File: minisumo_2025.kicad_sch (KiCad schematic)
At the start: 125 parts, among them J1 USB_C Connector, J10 DISTANCE_R90, J11 DISTANCE_R, J12 DISTANCE_RF, J13 DISTANCE_L90, J14 DISTANCE_L, J15 LINE_LEFT, J16 DISTANCE_LF, J3 START_MODULE, J4 MOTOR1, J5 MOTOR2, J6 BATT_IN, J8 DISTANCE_CENTER, J9 LINE_RIGHT, SW1 RESET, SW2 CASE, SW5 BOOT, U1 LMR33630ADDAR, U2 USBLC6-2P6, U3 ESP32-S3-WROOM-1, U4 TLV75733PDBVR, U5 TXS0108EPWR, U6 MC33926PNB, U7 MC33926PNB

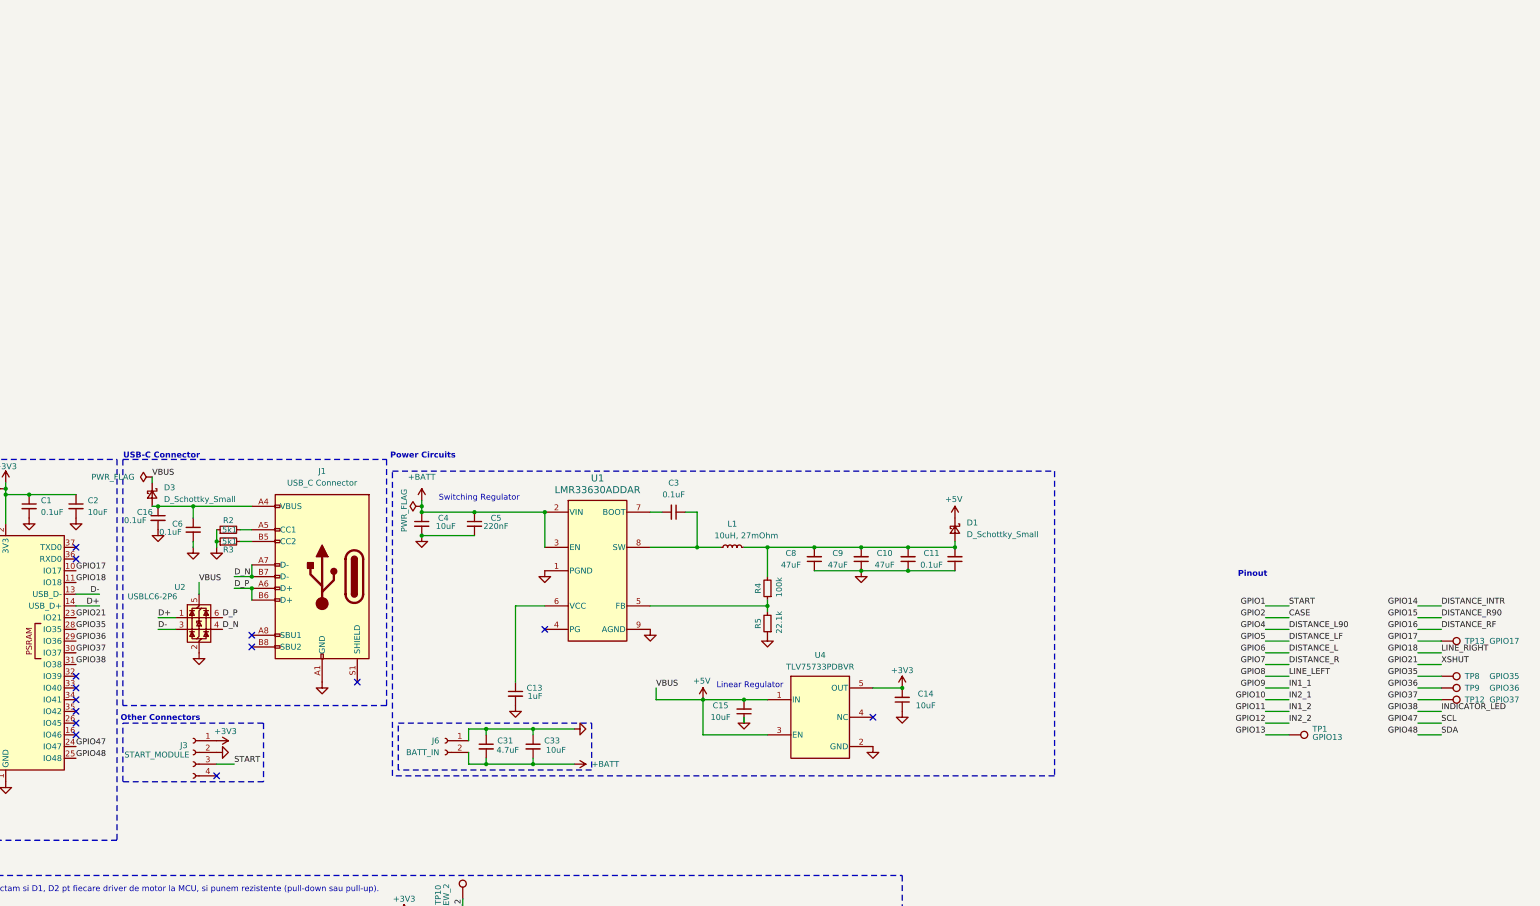
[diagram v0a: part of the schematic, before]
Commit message: final layout
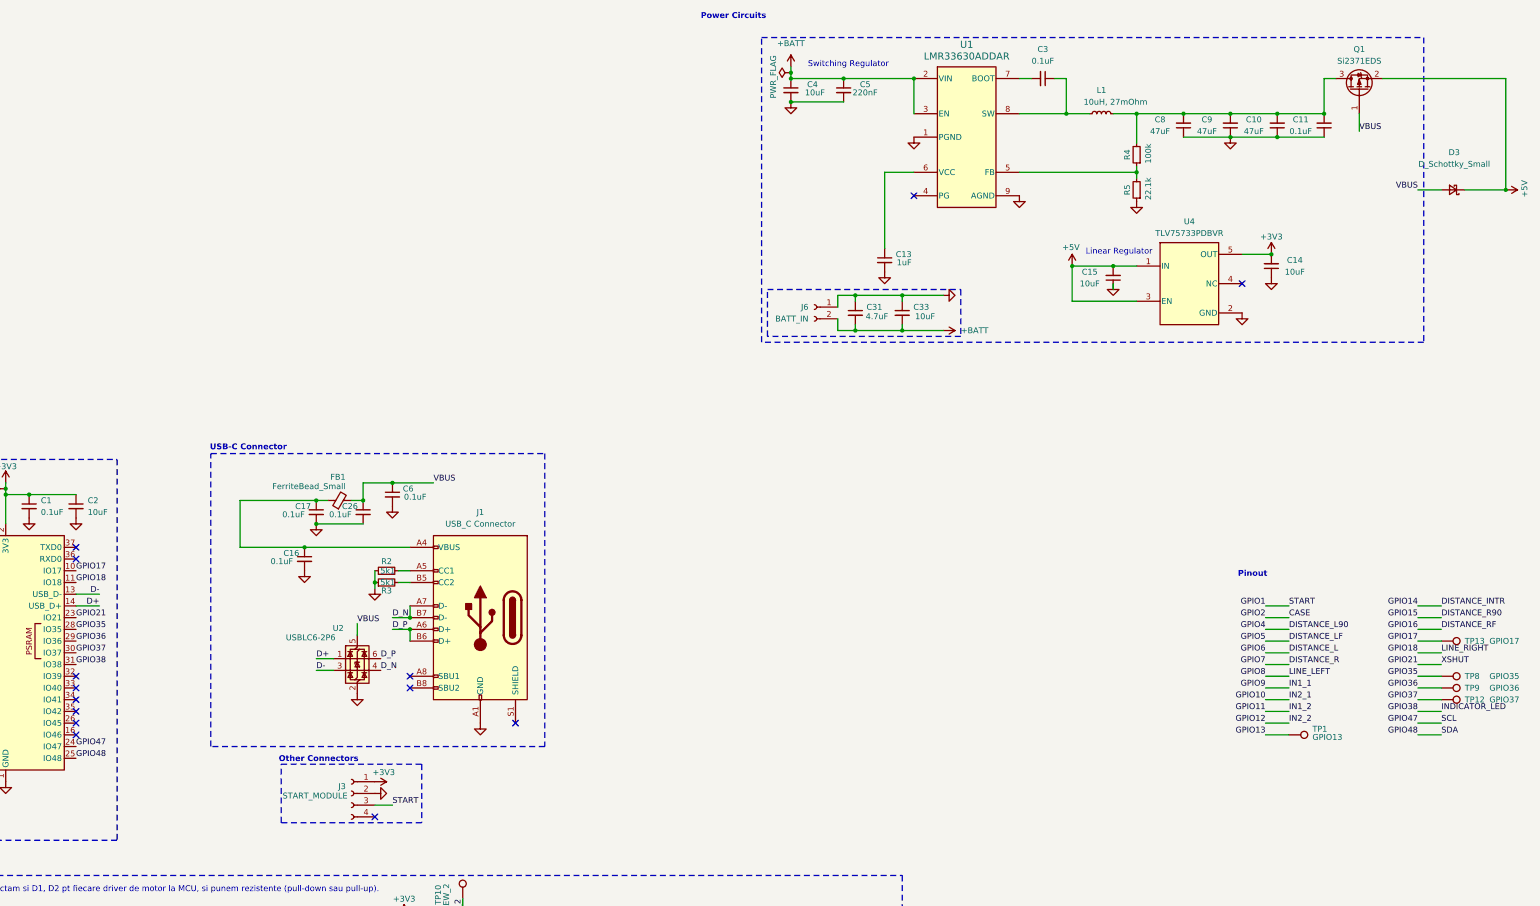
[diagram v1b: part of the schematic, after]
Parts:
- removed D1: D_Schottky_Small, Diode_SMD:D_SOD-123, symbol Device:D_Schottky_Small
- added C17, C26: 0.1uF, Capacitor_SMD:C_0603_1608Metric, symbol Device:C_Small
- added FB1: FerriteBead_Small, Capacitor_SMD:C_0805_2012Metric, symbol Device:FerriteBead_Small
- added Q1: Si2371EDS, Package_TO_SOT_SMD:SOT-23, symbol Transistor_FET:Si2371EDS
- D3: LCSC Part # C389355 -> (none)
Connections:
- net +5V: now also Q1.2 (S); no longer U2.5 (VBUS)
- net GND: now also C17.2, C26.2
- net at C10.2, C11.2, C8.2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: now also Q1.3 (D)
- net at C16.1, J1.A4 (VBUS), J1.A9 (VBUS)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: now also C17.1, FB1.1; no longer C6.1, D3.2 (A)
- new net VBUS: C26.1, C6.1, D3.2 (A), FB1.2, Q1.1 (G), U2.5 (VBUS)
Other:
- moved on the sheet: C10, C11, C13, C14, C15, C16, C3, C31, C33, C4, C5, C6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
